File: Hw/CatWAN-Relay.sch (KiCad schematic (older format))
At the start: 55 parts, among them J1 24v, J10 USB_B, J2 Output 3, J3 Input 1, J4 SWD, J5 Serial, J6 Output 2, J7 Output 1, J8 Input 2, J9 Input 3, Q1 MMBT2222A, Q2 MMBT2222A, Q3 MMBT2222A, SW1 RST, U1 ATSAMD21E, U2 RFM95W-868S2, U3 LTV-817, U4 LTV-817, U5 LTV-817, U6 LM2596_DC-DC, U7 AP2114H-3.3TRG1, Y1 UD2-3NU, Y2 UD2-3NU, Y3 UD2-3NU

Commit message: First route
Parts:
- removed J1: 24v, agroin:691313710002, symbol agroin-rescue:Conn_01x02
- removed J2: Output 3, agroin:691313710003, symbol agroin-rescue:Conn_01x03
- removed J3: Input 1, agroin:691313710003, symbol agroin-rescue:Conn_01x02
- removed J6: Output 2, agroin:691313710003, symbol agroin-rescue:Conn_01x03
- removed J7: Output 1, agroin:691313710003, symbol agroin-rescue:Conn_01x03
- removed J8: Input 2, agroin:691313710002, symbol agroin-rescue:Conn_01x02
- removed J9: Input 3, agroin:691313710002, symbol agroin-rescue:Conn_01x02
- removed MK1, MK2, MK3, MK4: Mounting_Hole, Mounting_Holes:MountingHole_3.5mm_Pad_Via, symbol agroin-rescue:Mounting_Hole
- added J2: INPUTS, TerminalBlock_Phoenix:TerminalBlock_Phoenix_MKDS-1,5-9-5.08_1x09_P5.08mm_Horizontal, symbol Connector:Conn_01x09_Female
- added J3: OUTPUTS, TerminalBlock_Phoenix:TerminalBlock_Phoenix_MKDS-1,5-9-5.08_1x09_P5.08mm_Horizontal, symbol Connector:Conn_01x09_Female
- AE1: footprint agroin:SMA_EDGE -> Connectors:MOLEX_1661; symbol agroin-rescue:Antenna_Shield -> CatWAN-Relay-rescue:Antenna_Shield-agroin-rescue
- C1, C3, C4, C5, C6, C7: footprint Capacitors_SMD:C_0805_HandSoldering -> Capacitor_SMD:C_0805_2012Metric_Pad1.15x1.40mm_HandSolder; symbol agroin-rescue:C -> CatWAN-Relay-rescue:C-agroin-rescue
- C2: footprint Capacitors_SMD:c_elec_6.3x7.7 -> Capacitor_SMD:C_Elec_6.3x7.7; symbol agroin-rescue:CP1 -> CatWAN-Relay-rescue:CP1-agroin-rescue
- D1, D2, D3: symbol agroin-rescue:FM4007W-W -> CatWAN-Relay-rescue:FM4007W-W-agroin-rescue
- D4: footprint Diodes_SMD:D_SOD-123 -> Diode_SMD:D_SOD-123; symbol agroin-rescue:FM4007W-W -> CatWAN-Relay-rescue:FM4007W-W-agroin-rescue
- D5: footprint Diodes_SMD:SOD-123 -> Diode_SMD:D_SOD-123; symbol agroin-rescue:MBR0520LT -> CatWAN-Relay-rescue:MBR0520LT-agroin-rescue
- D6, D7: footprint LEDs:LED_0805_HandSoldering -> LED_SMD:LED_0805_2012Metric_Pad1.15x1.40mm_HandSolder; symbol agroin-rescue:LED_Small -> CatWAN-Relay-rescue:LED_Small-agroin-rescue
- J10: symbol agroin-rescue:USB_B -> CatWAN-Relay-rescue:USB_B-agroin-rescue; manf# (none) -> 629105150521
- J4: footprint Pin_Headers:Pin_Header_Straight_1x04_Pitch2.54mm -> Connector_PinHeader_2.54mm:PinHeader_1x04_P2.54mm_Vertical; symbol agroin-rescue:Conn_01x04 -> CatWAN-Relay-rescue:Conn_01x04-agroin-rescue
- J5: footprint Pin_Headers:Pin_Header_Straight_1x03_Pitch2.54mm -> Connector_PinHeader_2.54mm:PinHeader_1x03_P2.54mm_Vertical; symbol agroin-rescue:Conn_01x03 -> CatWAN-Relay-rescue:Conn_01x03-agroin-rescue
- JP1: footprint Pin_Headers:Pin_Header_Straight_1x02_Pitch2.54mm -> Connector_PinHeader_2.54mm:PinHeader_1x02_P2.54mm_Vertical; symbol agroin-rescue:Jumper_NC_Small -> CatWAN-Relay-rescue:Jumper_NC_Small-agroin-rescue
- Q1, Q2, Q3: footprint TO_SOT_Packages_SMD:SOT-23 -> Package_TO_SOT_SMD:SOT-23; symbol agroin-rescue:MMBT2222A -> CatWAN-Relay-rescue:MMBT2222A-agroin-rescue
- R1, R10, R2, R3, R4, R5, R6, R7, R8: footprint Resistors_SMD:R_0805_HandSoldering -> Resistor_SMD:R_0805_2012Metric_Pad1.15x1.40mm_HandSolder; symbol agroin-rescue:R -> CatWAN-Relay-rescue:R-agroin-rescue
- R11, R9: footprint Resistors_SMD:R_0805_HandSoldering -> Resistor_SMD:R_0805_2012Metric_Pad1.15x1.40mm_HandSolder; symbol agroin-rescue:R_Small -> CatWAN-Relay-rescue:R_Small-agroin-rescue
- SW1: footprint Buttons_Switches_SMD:SW_SPST_B3U-1000P -> Button_Switch_SMD:SW_SPST_TL3342; symbol agroin-rescue:SW_Push -> CatWAN-Relay-rescue:SW_Push-agroin-rescue; manf# B3U-1000P -> -
- U1: footprint Housings_QFP:TQFP-32_7x7mm_Pitch0.8mm -> Package_QFP:TQFP-32_7x7mm_P0.8mm; symbol agroin-rescue:ATSAMD21E -> CatWAN-Relay-rescue:ATSAMD21E-agroin-rescue
- U2: symbol agroin-rescue:RFM95W-868S2 -> CatWAN-Relay-rescue:RFM95W-868S2-agroin-rescue; Field4 RFM95W-868S2 -> (none); Field5 Warning -> (none); Field6 7.22 USD -> (none); Field7 RF -> (none)
- U3, U4, U5: footprint Housings_DIP:DIP-4_W7.62mm -> Package_DIP:DIP-4_W7.62mm_Socket; symbol agroin-rescue:LTV-817 -> CatWAN-Relay-rescue:LTV-817-agroin-rescue
- U6: symbol agroin-rescue:LM2596_DC-DC -> CatWAN-Relay-rescue:LM2596_DC-DC-agroin-rescue
- U7: footprint TO_SOT_Packages_SMD:SOT-223-3Lead_TabPin2 -> Package_TO_SOT_SMD:SOT-223-3_TabPin2; symbol agroin-rescue:AP2114H-3.3TRG1 -> CatWAN-Relay-rescue:AP2114H-3.3TRG1-agroin-rescue
- Y1, Y2, Y3: symbol agroin-rescue:UD2-3NU -> CatWAN-Relay-rescue:UD2-3NU-agroin-rescue
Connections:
- wire segments 144 -> 147

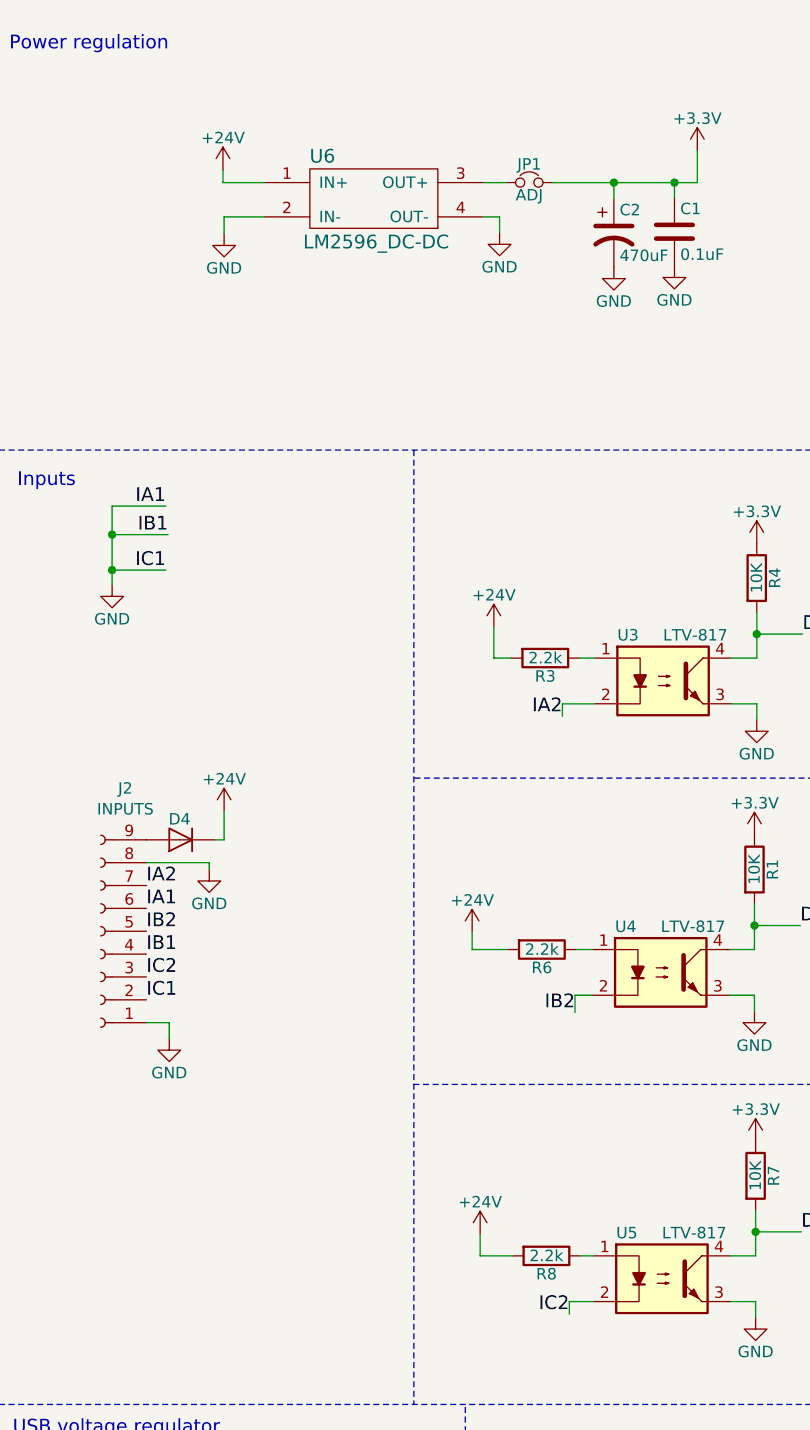
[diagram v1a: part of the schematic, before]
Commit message: Add_Diode
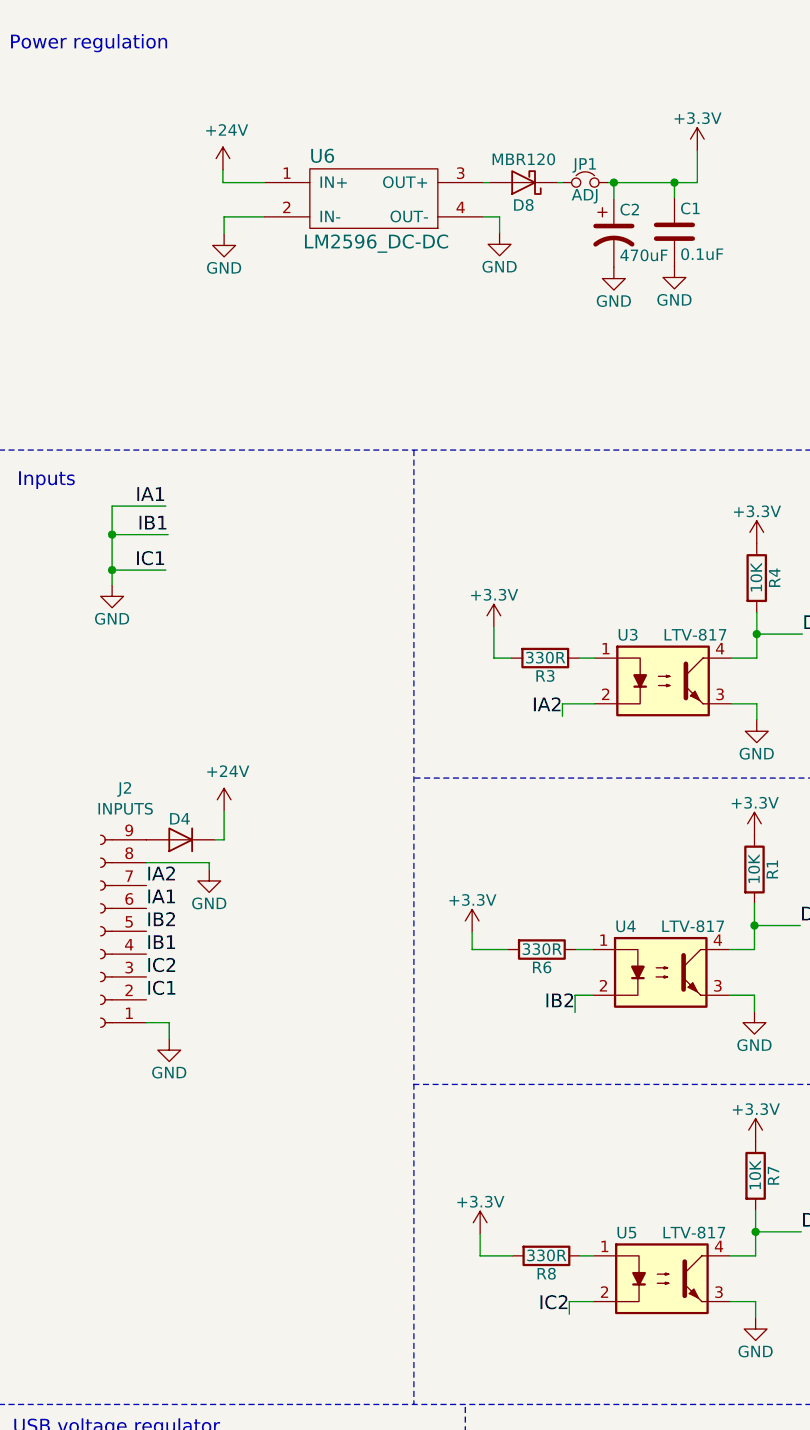
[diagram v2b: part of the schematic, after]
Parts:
- added D8: MBR120, Diode_SMD:D_SOD-123, symbol CatWAN-Relay-rescue:MBR0520LT-agroin-rescue
- R3, R6, R8: value 2.2k -> 330R
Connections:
- net +24V: no longer R3.2, R6.2, R8.2
- net +3V3: now also R3.2, R6.2, R8.2
- net at JP1.1: now also D8.1 (K); no longer U6.3 (OUT+)
- new net: D8.2 (A), U6.3 (OUT+)
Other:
- moved on the sheet: JP1
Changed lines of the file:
@@
 EESchema Schematic File Version 4
-LIBS:CatWAN-Relay-cache
-EELAYER 29 0
+EELAYER 30 0
 EELAYER END
 $Descr A4 11693 8268
@@
 $EndComp
 $Comp
-L CatWAN-Relay-rescue:Jumper_NC_Small-agroin-rescue JP1
-U 1 1 5AE4CD32
-P 2795 1195
-F 0 "JP1" H 2795 1275 50  0000 C CNN
-F 1 "ADJ" H 2795 1140 50  0000 C CNN
-F 2 "Connector_PinHeader_2.54mm:PinHeader_1x02_P2.54mm_Vertical" H 2795 1195 50  0001 C CNN
-F 3 "" H 2795 1195 50  0001 C CNN
-	1    2795 1195
-	1    0    0    -1
-$EndComp
-$Comp
 L CatWAN-Relay-rescue:C-agroin-rescue C1
 U 1 1 5AE4C7D8
@@
 Text Label 1120 4470 0    60   ~ 0
 IB2
-$Comp
-L CatWAN-Relay-rescue:R-agroin-rescue R3
-U 1 1 5AE7BE19
-P 2865 3275
-F 0 "R3" V 2945 3275 50  0000 C CNN
-F 1 "2.2k" V 2865 3275 50  0000 C CNN
-F 2 "Resistor_SMD:R_0805_2012Metric_Pad1.15x1.40mm_HandSolder" V 2795 3275 50  0001 C CNN
-F 3 "" H 2865 3275 50  0001 C CNN
-F 4 "CRCW08052K20FKEB" V 2865 3275 60  0001 C CNN "manf#"
-	1    2865 3275
-	0    1    1    0
-$EndComp
 Text Label 1120 4270 0    60   ~ 0
 IA2
@@
 IC1
 $Comp
-L CatWAN-Relay-rescue:+24V-agroin-rescue #PWR014
-U 1 1 5AE7DFDE
-P 1455 1140
-F 0 "#PWR014" H 1455 990 50  0001 C CNN
-F 1 "+24V" H 1455 1280 50  0000 C CNN
-F 2 "" H 1455 1140 50  0001 C CNN
-F 3 "" H 1455 1140 50  0001 C CNN
-	1    1455 1140
-	1    0    0    -1
-$EndComp
-$Comp
-L CatWAN-Relay-rescue:+24V-agroin-rescue #PWR015
-U 1 1 5AE7E111
-P 1460 3945
-F 0 "#PWR015" H 1460 3795 50  0001 C CNN
-F 1 "+24V" H 1460 4085 50  0000 C CNN
-F 2 "" H 1460 3945 50  0001 C CNN
-F 3 "" H 1460 3945 50  0001 C CNN
-	1    1460 3945
-	1    0    0    -1
-$EndComp
-$Comp
-L CatWAN-Relay-rescue:+24V-agroin-rescue #PWR016
-U 1 1 5AE7EE53
-P 2640 3140
-F 0 "#PWR016" H 2640 2990 50  0001 C CNN
-F 1 "+24V" H 2640 3280 50  0000 C CNN
-F 2 "" H 2640 3140 50  0001 C CNN
-F 3 "" H 2640 3140 50  0001 C CNN
-	1    2640 3140
-	1    0    0    -1
-$EndComp
-$Comp
 L CatWAN-Relay-rescue:+3.3V-agroin-rescue #PWR017
 U 1 1 5AE7FC5E
@@
 	2665 1345 2595 1345
 Wire Wire Line
-	2595 1195 2695 1195
-Wire Wire Line
-	2895 1195 3165 1195
-Wire Wire Line
 	3430 1195 3430 1260
 Wire Wire Line
 	3165 1195 3165 1265
-Connection ~ 3165 1195
 Wire Wire Line
 	3530 1195 3530 1055
@@
 Wire Wire Line
 	2940 3475 3080 3475
-Wire Wire Line
-	1455 1195 1455 1140
 Wire Wire Line
 	1460 1420 1460 1345
@@
 	1    0    0    -1
 $EndComp
-$Comp
-L CatWAN-Relay-rescue:R-agroin-rescue R6
-U 1 1 5B076E84
-P 2850 4550
-F 0 "R6" V 2930 4550 50  0000 C CNN
-F 1 "2.2k" V 2850 4550 50  0000 C CNN
-F 2 "Resistor_SMD:R_0805_2012Metric_Pad1.15x1.40mm_HandSolder" V 2780 4550 50  0001 C CNN
-F 3 "" H 2850 4550 50  0001 C CNN
-F 4 "CRCW08052K20FKEB" V 2850 4550 60  0001 C CNN "manf#"
-	1    2850 4550
-	0    1    1    0
-$EndComp
 Text Label 2995 4825 2    60   ~ 0
 IB2
@@
 	1    3375 5990
 	1    0    0    -1
-$EndComp
-$Comp
-L CatWAN-Relay-rescue:R-agroin-rescue R8
-U 1 1 5B076F9E
-P 2870 5890
-F 0 "R8" V 2950 5890 50  0000 C CNN
-F 1 "2.2k" V 2870 5890 50  0000 C CNN
-F 2 "Resistor_SMD:R_0805_2012Metric_Pad1.15x1.40mm_HandSolder" V 2800 5890 50  0001 C CNN
-F 3 "" H 2870 5890 50  0001 C CNN
-F 4 "CRCW08052K20FKEB" V 2870 5890 60  0001 C CNN "manf#"
-	1    2870 5890
-	0    1    1    0
 $EndComp
 Text Label 2970 6145 2    60   ~ 0
@@
 	2715 3275 2640 3275
 Wire Wire Line
-	2640 3275 2640 3140
-Wire Wire Line
 	970  2610 1205 2610
 Wire Wire Line
 	1215 2735 970  2735
 Connection ~ 970  2735
-$Comp
-L CatWAN-Relay-rescue:+24V-agroin-rescue #PWR047
-U 1 1 5B0CD439
-P 2545 4475
-F 0 "#PWR047" H 2545 4325 50  0001 C CNN
-F 1 "+24V" H 2545 4615 50  0000 C CNN
-F 2 "" H 2545 4475 50  0001 C CNN
-F 3 "" H 2545 4475 50  0001 C CNN
-	1    2545 4475
-	1    0    0    -1
-$EndComp
 Wire Wire Line
 	2700 4550 2545 4550
 Wire Wire Line
 	2545 4550 2545 4475
-$Comp
-L CatWAN-Relay-rescue:+24V-agroin-rescue #PWR048
-U 1 1 5B0CE393
-P 2580 5795
-F 0 "#PWR048" H 2580 5645 50  0001 C CNN
-F 1 "+24V" H 2580 5935 50  0000 C CNN
-F 2 "" H 2580 5795 50  0001 C CNN
-F 3 "" H 2580 5795 50  0001 C CNN
-	1    2580 5795
-	1    0    0    -1
-$EndComp
 Wire Wire Line
 	2720 5890 2580 5890
@@
 	1    0    0    -1
 $EndComp
+Wire Wire Line
+	1455 1140 1455 1195
+Wire Wire Line
+	2640 3140 2640 3275
+$Comp
+L CatWAN-Relay-rescue:+3.3V-agroin-rescue #PWR047
+U 1 1 5F877236
+P 2640 3140
+F 0 "#PWR047" H 2640 2990 50  0001 C CNN
+F 1 "+3.3V" H 2640 3280 50  0000 C CNN
+F 2 "" H 2640 3140 50  0001 C CNN
+F 3 "" H 2640 3140 50  0001 C CNN
+	1    2640 3140
+	1    0    0    -1
+$EndComp
+$Comp
+L CatWAN-Relay-rescue:+3.3V-agroin-rescue #PWR016
+U 1 1 5F879B69
+P 2545 4475
+F 0 "#PWR016" H 2545 4325 50  0001 C CNN
+F 1 "+3.3V" H 2545 4615 50  0000 C CNN
+F 2 "" H 2545 4475 50  0001 C CNN
+F 3 "" H 2545 4475 50  0001 C CNN
+	1    2545 4475
+	1    0    0    -1
+$EndComp
+$Comp
+L CatWAN-Relay-rescue:+3.3V-agroin-rescue #PWR035
+U 1 1 5F87A3E3
+P 2580 5795
+F 0 "#PWR035" H 2580 5645 50  0001 C CNN
+F 1 "+3.3V" H 2580 5935 50  0000 C CNN
+F 2 "" H 2580 5795 50  0001 C CNN
+F 3 "" H 2580 5795 50  0001 C CNN
+	1    2580 5795
+	1    0    0    -1
+$EndComp
+$Comp
+L CatWAN-Relay-rescue:R-agroin-rescue R8
+U 1 1 5B076F9E
+P 2870 5890
+F 0 "R8" V 2950 5890 50  0000 C CNN
+F 1 "330R" V 2870 5890 50  0000 C CNN
+F 2 "Resistor_SMD:R_0805_2012Metric_Pad1.15x1.40mm_HandSolder" V 2800 5890 50  0001 C CNN
+F 3 "" H 2870 5890 50  0001 C CNN
+F 4 "CRCW08052K20FKEB" V 2870 5890 60  0001 C CNN "manf#"
+	1    2870 5890
+	0    1    1    0
+$EndComp
+$Comp
+L CatWAN-Relay-rescue:R-agroin-rescue R6
+U 1 1 5B076E84
+P 2850 4550
+F 0 "R6" V 2930 4550 50  0000 C CNN
+F 1 "330R" V 2850 4550 50  0000 C CNN
+F 2 "Resistor_SMD:R_0805_2012Metric_Pad1.15x1.40mm_HandSolder" V 2780 4550 50  0001 C CNN
+F 3 "" H 2850 4550 50  0001 C CNN
+F 4 "CRCW08052K20FKEB" V 2850 4550 60  0001 C CNN "manf#"
+	1    2850 4550
+	0    1    1    0
+$EndComp
+$Comp
+L CatWAN-Relay-rescue:R-agroin-rescue R3
+U 1 1 5AE7BE19
+P 2865 3275
+F 0 "R3" V 2945 3275 50  0000 C CNN
+F 1 "330R" V 2865 3275 50  0000 C CNN
+F 2 "Resistor_SMD:R_0805_2012Metric_Pad1.15x1.40mm_HandSolder" V 2795 3275 50  0001 C CNN
+F 3 "" H 2865 3275 50  0001 C CNN
+F 4 "CRCW08052K20FKEB" V 2865 3275 60  0001 C CNN "manf#"
+	1    2865 3275
+	0    1    1    0
+$EndComp
+$Comp
+L CatWAN-Relay-rescue:Jumper_NC_Small-agroin-rescue JP1
+U 1 1 5AE4CD32
+P 3040 1195
+F 0 "JP1" H 3040 1275 50  0000 C CNN
+F 1 "ADJ" H 3040 1140 50  0000 C CNN
+F 2 "Connector_PinHeader_2.54mm:PinHeader_1x02_P2.54mm_Vertical" H 3040 1195 50  0001 C CNN
+F 3 "" H 3040 1195 50  0001 C CNN
+	1    3040 1195
+	1    0    0    -1
+$EndComp
+Wire Wire Line
+	3140 1195 3165 1195
+Connection ~ 3165 1195
+$Comp
+L CatWAN-Relay-rescue:MBR0520LT-agroin-rescue D8
+U 1 1 5F87B0CE
+P 2770 1195
+F 0 "D8" H 2770 1295 50  0000 C CNN
+F 1 "MBR120" H 2770 1095 50  0000 C CNN
+F 2 "Diode_SMD:D_SOD-123" H 2770 1020 50  0001 C CNN
+F 3 "" H 2770 1195 50  0001 C CNN
+F 4 "MBR120VLSFT3G" H 2770 1195 60  0001 C CNN "manf#"
+	1    2770 1195
+	-1   0    0    1
+$EndComp
+Wire Wire Line
+	2595 1195 2620 1195
+Wire Wire Line
+	2920 1195 2940 1195
+$Comp
+L power:+24V #PWR0104
+U 1 1 5F8FD38D
+P 1455 1140
+F 0 "#PWR0104" H 1455 990 50  0001 C CNN
+F 1 "+24V" H 1470 1313 50  0000 C CNN
+F 2 "" H 1455 1140 50  0001 C CNN
+F 3 "" H 1455 1140 50  0001 C CNN
+	1    1455 1140
+	1    0    0    -1
+$EndComp
+$Comp
+L power:+24V #PWR0103
+U 1 1 5F904D47
+P 1460 3945
+F 0 "#PWR0103" H 1460 3795 50  0001 C CNN
+F 1 "+24V" H 1475 4118 50  0000 C CNN
+F 2 "" H 1460 3945 50  0001 C CNN
+F 3 "" H 1460 3945 50  0001 C CNN
+	1    1460 3945
+	1    0    0    -1
+$EndComp
